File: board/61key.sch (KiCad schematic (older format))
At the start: 147 parts, among them J1 105450-0101, J10 Conn_01x01_Male, J11 Conn_01x01_Male, J12 Conn_01x01_Male, J13 Conn_01x01_Male, J2 Conn_01x01_Male, J3 Conn_01x01_Male, J4 Conn_01x01_Male, J5 Conn_01x01_Male, J6 Conn_01x01_Male, J7 Conn_01x01_Male, J8 Conn_01x01_Male, J9 Conn_01x01_Male, SW1 SW_SPST, SW10 SW_SPST, SW11 SW_SPST, SW12 SW_SPST, SW13 SW_SPST, SW14 SW_SPST, SW15 SW_SPST, SW16 SW_SPST, SW17 SW_SPST, SW18 SW_SPST, SW19 SW_SPST, SW2 SW_SPST, SW20 SW_SPST, SW21 SW_SPST, SW22 SW_SPST, SW23 SW_SPST, SW24 SW_SPST, SW25 SW_SPST, SW26 SW_SPST, SW27 SW_SPST, SW28 SW_SPST, SW29 SW_SPST, SW3 SW_SPST, SW30 SW_SPST, SW31 SW_SPST, SW32 SW_SPST, SW33 SW_SPST, SW34 SW_SPST, SW35 SW_SPST, SW36 SW_SPST, SW37 SW_SPST, SW38 SW_SPST, SW39 SW_SPST, SW4 SW_SPST, SW40 SW_SPST, SW41 SW_SPST, SW42 SW_SPST, SW43 SW_SPST, SW44 SW_SPST, SW45 SW_SPST, SW46 SW_SPST, SW47 SW_SPST, SW48 SW_SPST, SW49 SW_SPST, SW5 SW_SPST, SW50 SW_SPST, SW51 SW_SPST, SW52 SW_SPST, SW53 SW_SPST, SW54 SW_SPST, SW55 SW_SPST, SW56 SW_SPST, SW57 SW_SPST, SW58 SW_SPST, SW59 SW_SPST, SW6 SW_SPST, SW60 SW_SPST, SW61 SW_SPST, SW7 SW_SPST, SW8 SW_SPST, SW9 SW_SPST, U1 ATmega32U4-AU, X1 FA-238

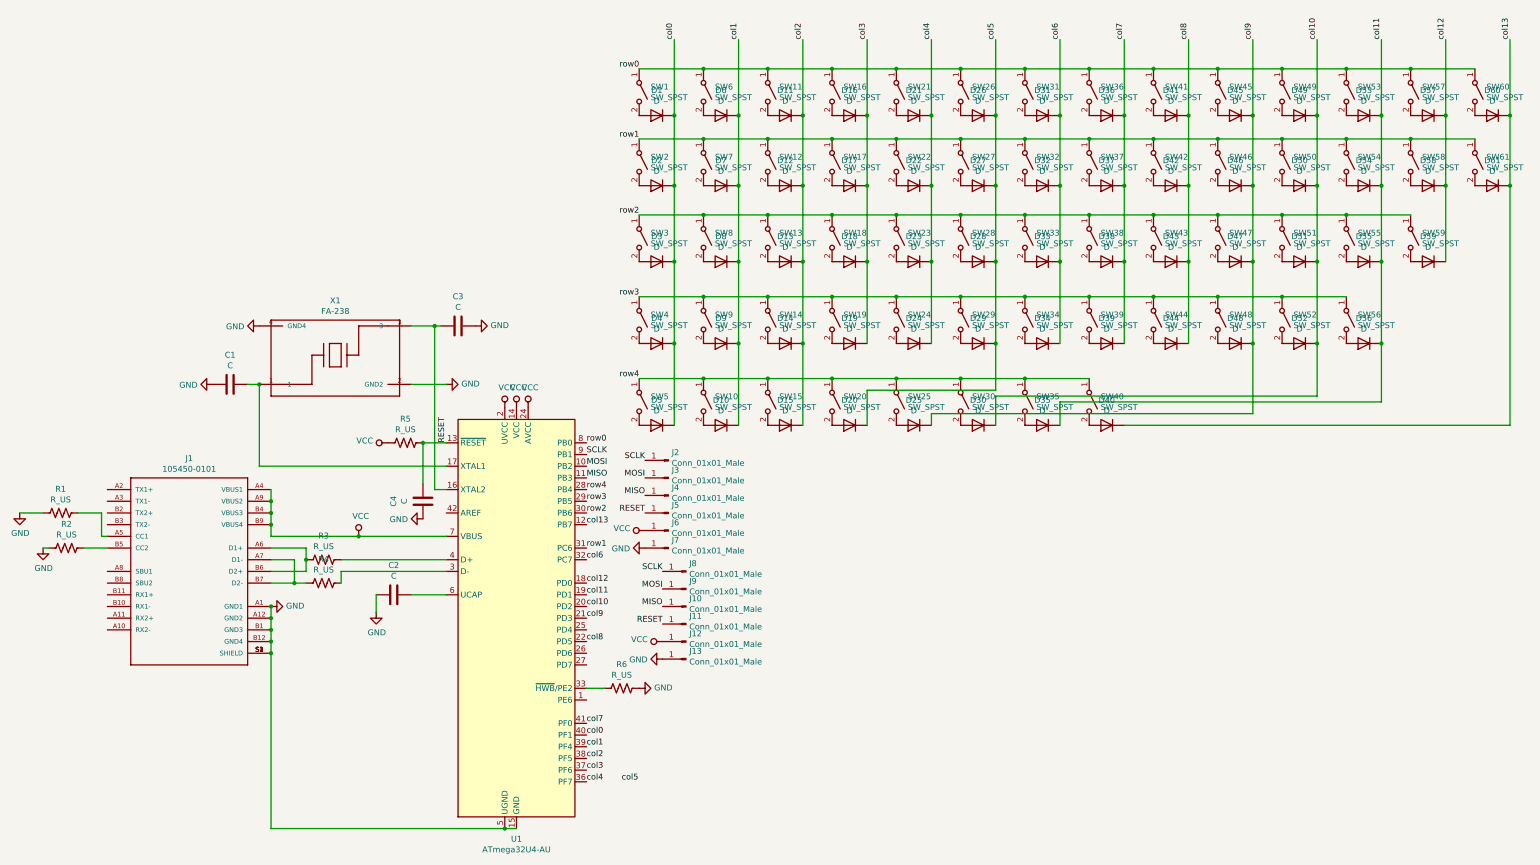
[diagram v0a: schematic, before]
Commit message: big overhaul
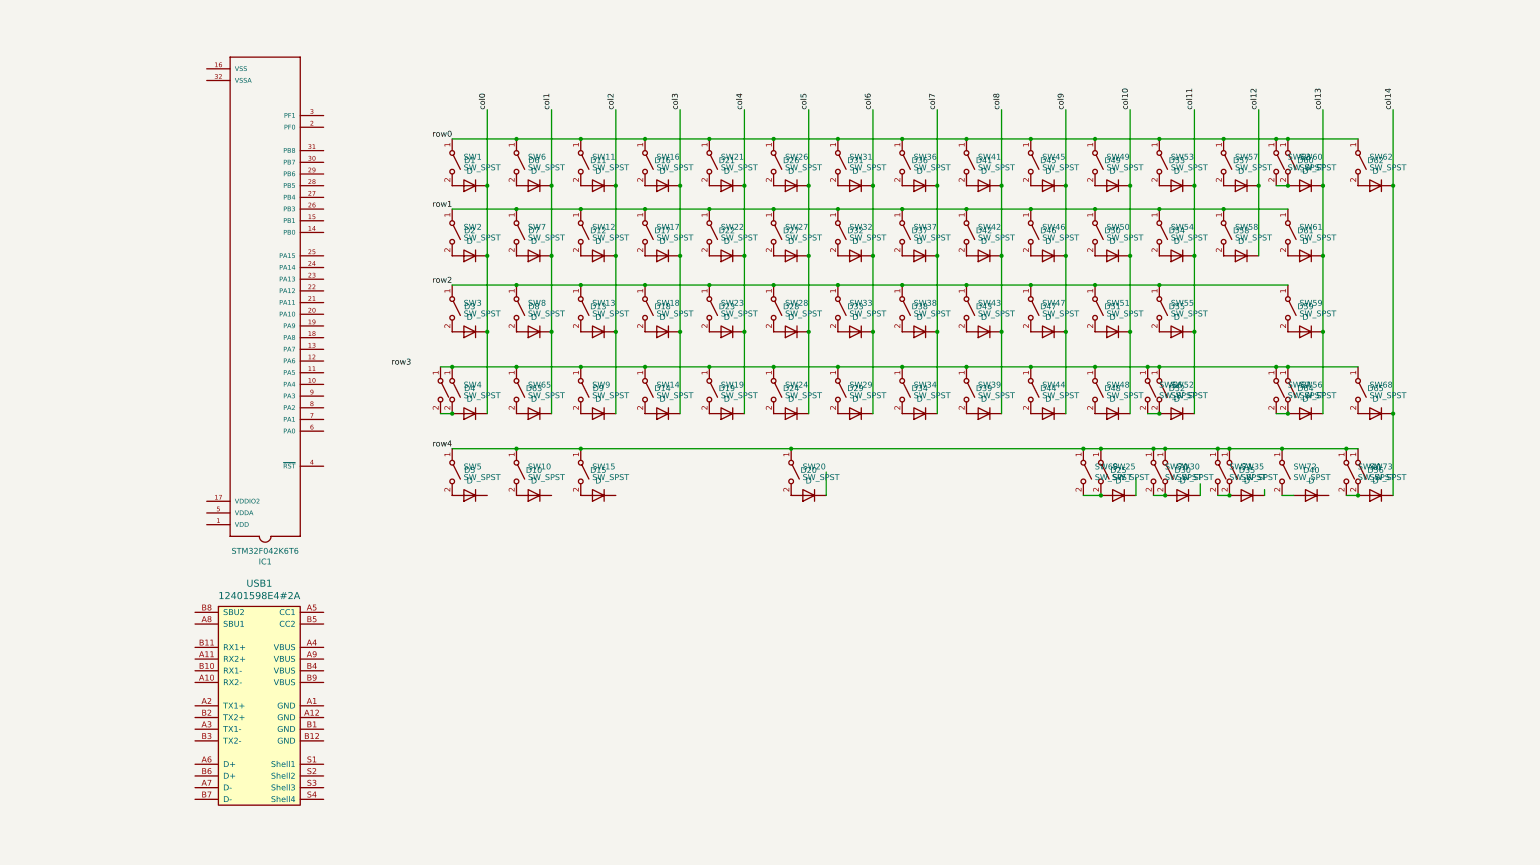
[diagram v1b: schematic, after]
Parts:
- removed C1, C2, C3, C4: C, Capacitor_SMD:C_0805_2012Metric, symbol Device:C
- removed J1: 105450-0101, 61key:MOLEX_105450-0101, symbol 61key:105450-0101
- removed J10, J11, J12, J13, J2, J3, J4, J5, J6, J7, J8, J9: Conn_01x01_Male, 61key:pad-nosilk, symbol Connector:Conn_01x01_Male
- removed R1, R2, R3, R4, R5, R6: R_US, Resistor_SMD:R_0805_2012Metric, symbol Device:R_US
- removed U1: ATmega32U4-AU, 61key:QFN-44-1EP_7x7mm_Pitch0.5mm, symbol MCU_Microchip_ATmega:ATmega32U4-AU
- removed X1: FA-238, 61key:OSCCC320X250X70-4N, symbol 61key:FA-238
- added D62, D63, D64, D65: D, 61key:D_0805_2012Metric, symbol Device:D
- added IC1: STM32F042K6T6, symbol 61key:STM32F042K6T6
- added SW62, SW63, SW64, SW65, SW66, SW67, SW68, SW69, SW70, SW71, SW72, SW73: SW_SPST, 61key:SW_MX, symbol Switch:SW_SPST
- added USB1: 12401598E4#2A, symbol 61key:12401598E4#2A
- SW1, SW11, SW12, SW13, SW14, SW16, SW17, SW18, SW19, SW21, SW22, SW23, SW24, SW26, SW27, SW28, SW29, SW31, SW32, SW33, SW34, SW36, SW37, SW38, SW39, SW41, SW42, SW43, SW44, SW45, SW46, SW47, SW48, SW49, SW50, SW51, SW52, SW53, SW54, SW55, SW57, SW58, SW6, SW7, SW8, SW9: footprint 61key:MX-1U-NoLED -> 61key:SW_MX
- SW10, SW15, SW25, SW30, SW35, SW40, SW5: footprint 61key:MX-1.25U-NoLED -> 61key:SW_MX
- SW2, SW61: footprint 61key:MX-1.5U-NoLED -> 61key:SW_MX
- SW20: footprint 61key:MX-6.25U-NoLED -> 61key:SW_MX
- SW3: footprint 61key:MX-1.75U-NoLED -> 61key:SW_MX
- SW4, SW59: footprint 61key:MX-2.25U-NoLED -> 61key:SW_MX
- SW56: footprint 61key:MX-2.75U-NoLED -> 61key:SW_MX
- SW60: footprint 61key:MX-2U-NoLED -> 61key:SW_MX
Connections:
- net labels added: col14
- net labels removed: GND, MISO, MOSI, RESET, SCLK, VCC
- wire segments 169 -> 138
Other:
- moved on the sheet: D1, D10, D11, D12, D13, D14, D15, D16, D17, D18, D19, D2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
